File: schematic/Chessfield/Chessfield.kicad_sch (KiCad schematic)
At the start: 13 parts, among them J1 Conn_01x04_Pin, J2 Conn_01x04_Pin, J3 Conn_01x04_Pin, J4 Conn_01x04_Pin

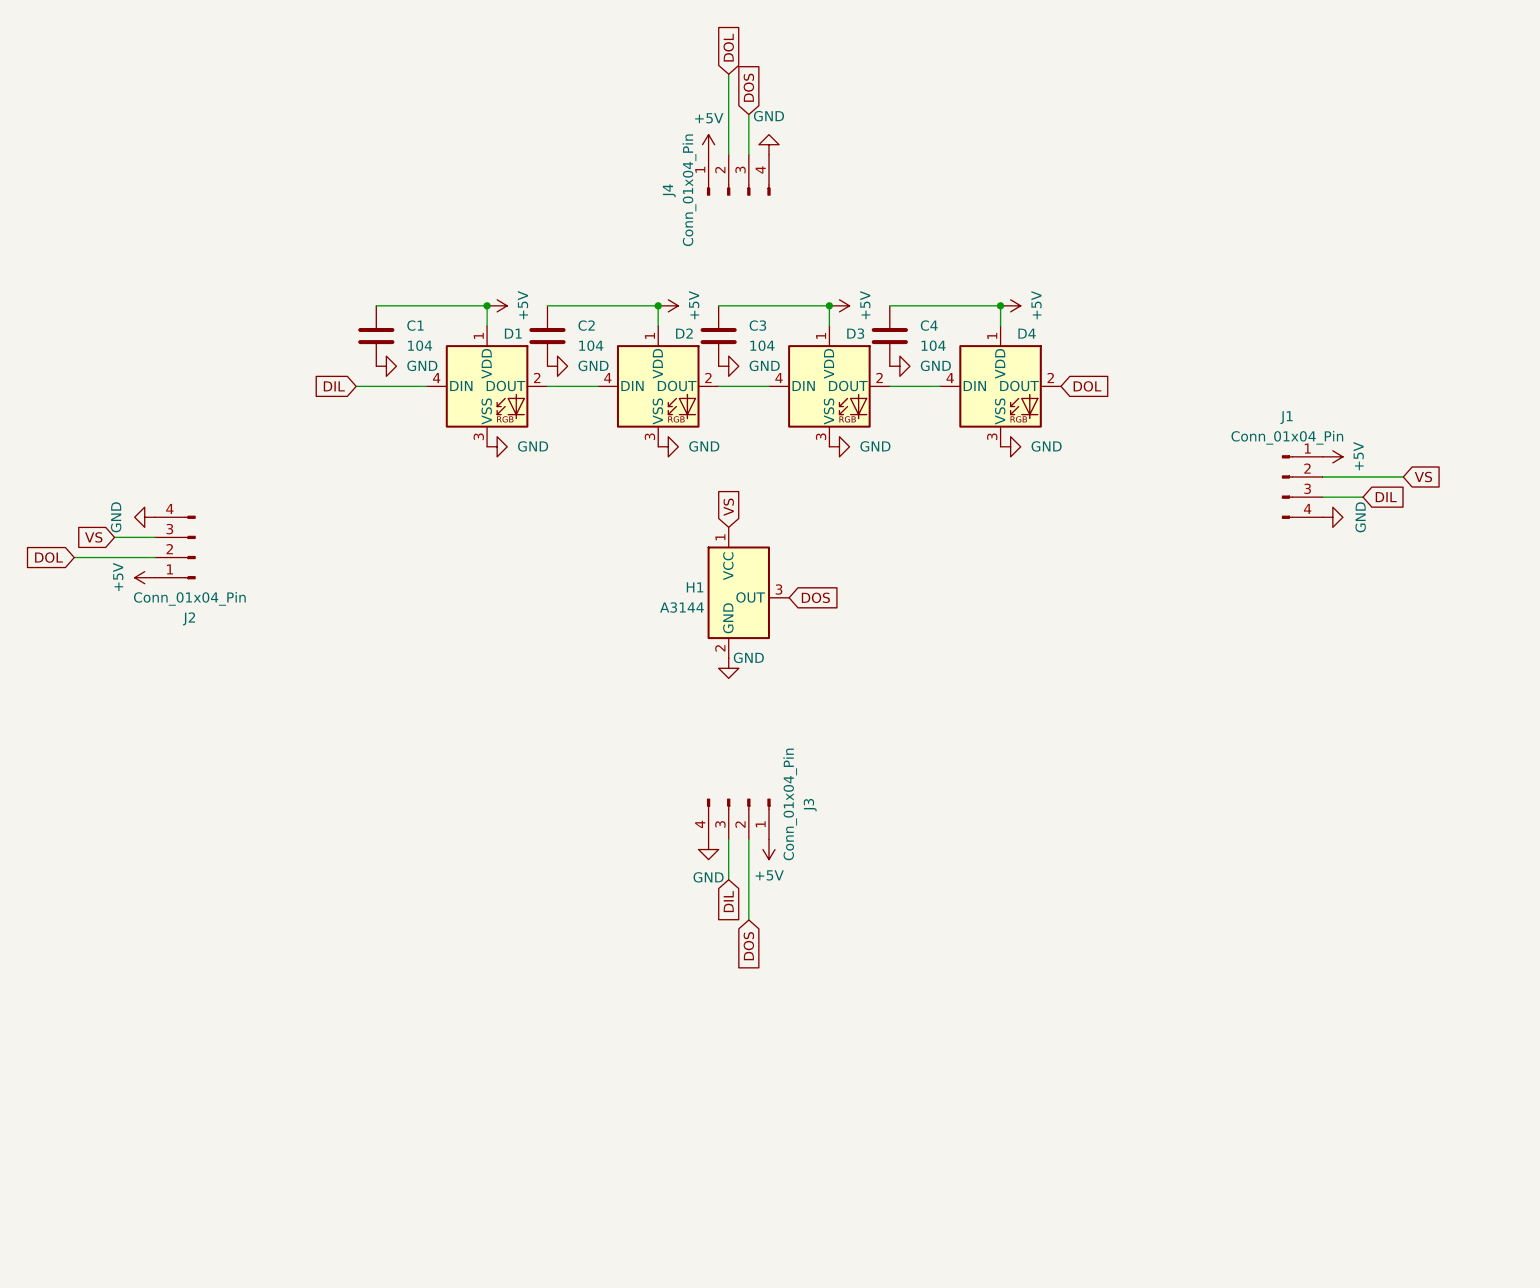
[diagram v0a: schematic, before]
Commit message: finish chessfield
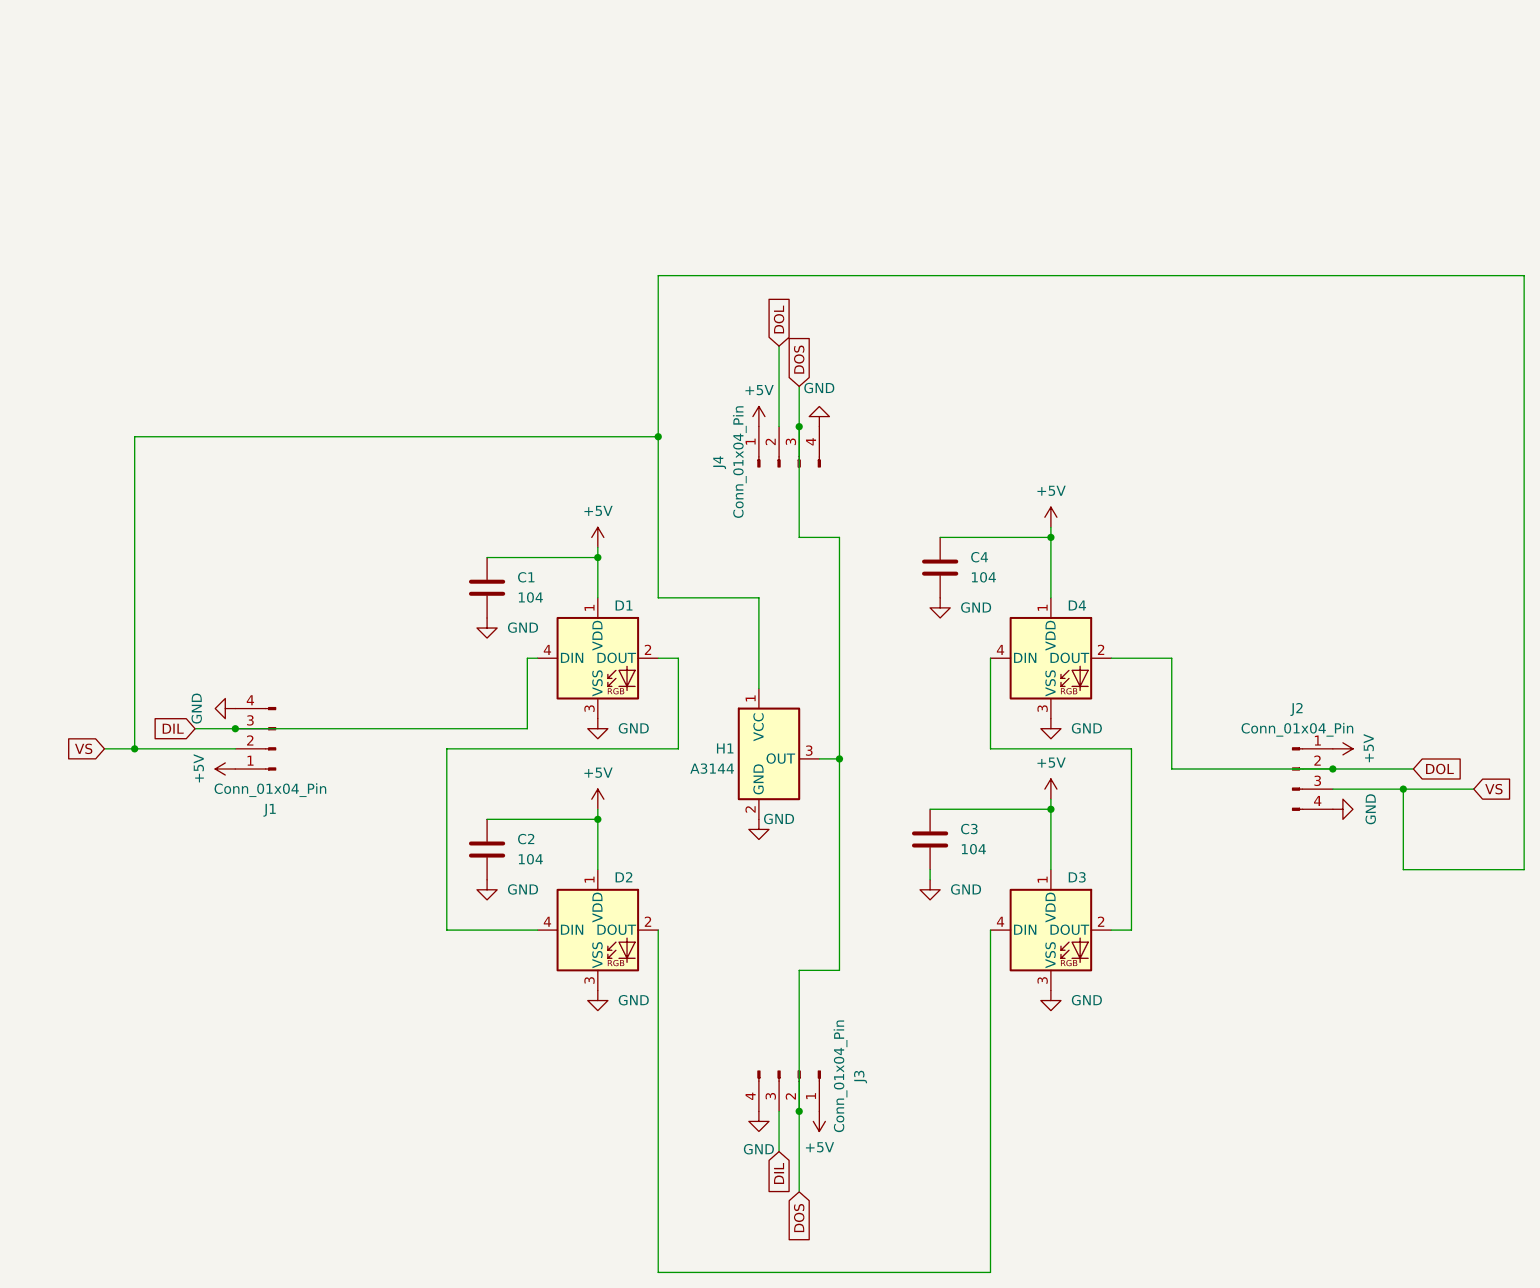
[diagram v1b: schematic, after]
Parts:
- H1: footprint Package_TO_SOT_THT:TO-92_Inline -> Package_TO_SOT_THT:TO-92_Inline_Horizontal1
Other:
- moved on the sheet: C1, C2, C3, C4, D1, D2, D3, D4, H1, J1, J2, J3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
